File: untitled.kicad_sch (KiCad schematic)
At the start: 4 parts

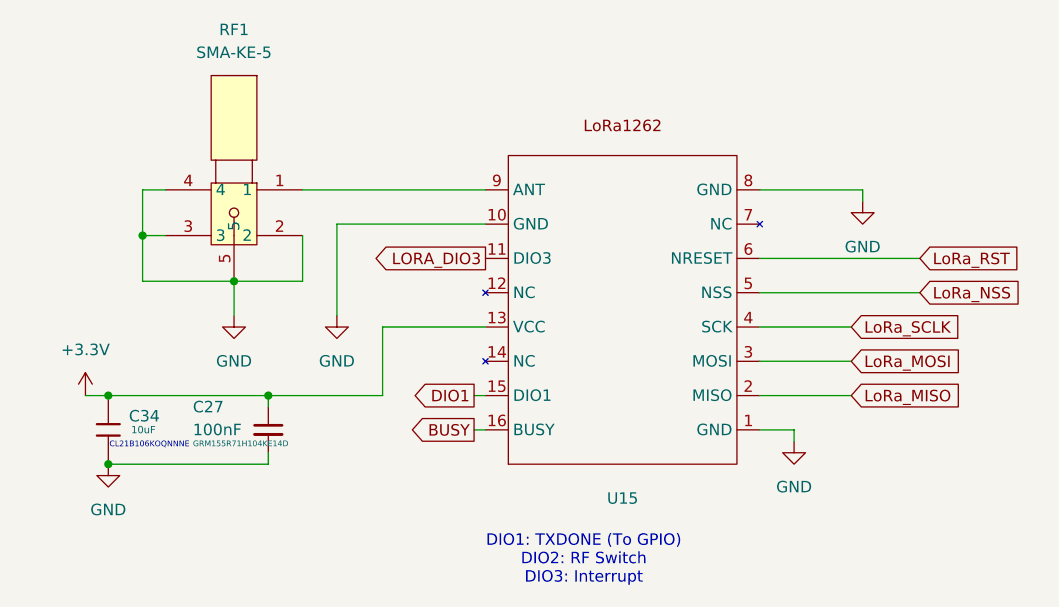
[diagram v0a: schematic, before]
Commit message: Chore: push new design
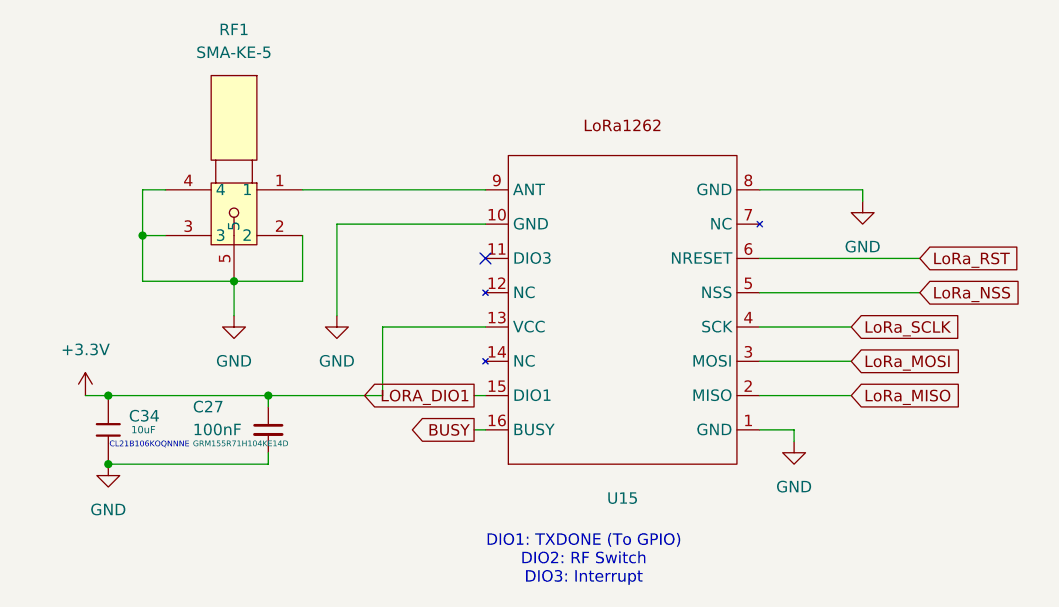
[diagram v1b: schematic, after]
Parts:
- C27, C34: footprint PCM_JLCPCB:C_0402 -> PCM_JLCPCB:C_0603
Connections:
- net DIO1 renamed LORA_DIO1
- net LORA_DIO3: no longer names the net of U15.11 (DIO3)
- no-connect marks 0 -> 1

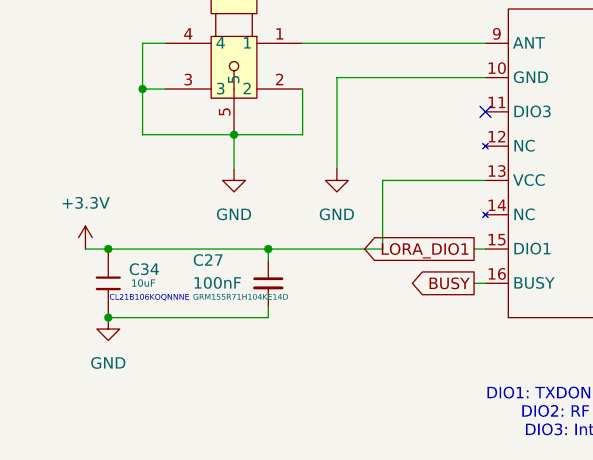
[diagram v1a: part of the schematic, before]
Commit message: Special version
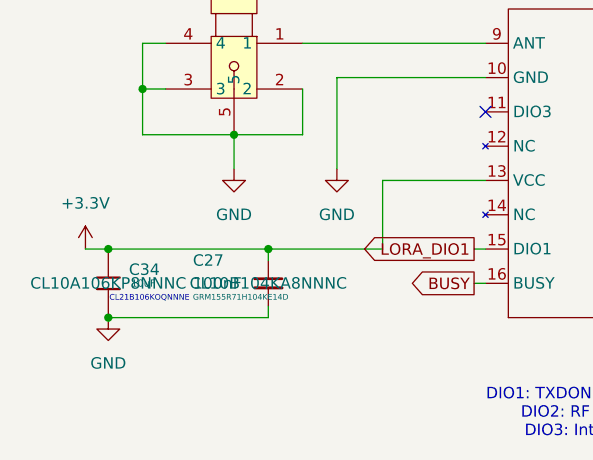
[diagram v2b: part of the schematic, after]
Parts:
- C27: Digikey Parts (none) -> CL10B104KA8NNNC
- C34: Digikey Parts (none) -> CL10A106KP8NNNC
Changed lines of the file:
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@@
+			)
+		)
+		(property "Digikey Parts" "CL10B104KA8NNNC"
+			(at 81.28 100.33 0)
+			(effects
+				(font
+					(size 1.27 1.27)
+				)
 			)
 		)
@@
 		)
 		(property "Sim.Pins" ""
+			(at 63.5 100.33 0)
+			(effects
+				(font
+					(size 1.27 1.27)
+				)
+			)
+		)
+		(property "Digikey Parts" "CL10A106KP8NNNC"
 			(at 63.5 100.33 0)
 			(effects
@@
 			)
 		)
+		(property "Digikey Parts" ""
+			(at 77.47 73.66 0)
+			(effects
+				(font
+					(size 1.27 1.27)
+				)
+			)
+		)
 		(pin "5"
 		)
@@
 			(at 120.65 69.85 0)
 			(effects
+				(font
+					(size 1.27 1.27)
+				)
+			)
+		)
+		(property "Digikey Parts" ""
+			(at 120.65 69.85 0)
+			(effects
